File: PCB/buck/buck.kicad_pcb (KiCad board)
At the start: 2 copper layers, 30 x 27 mm, 7 parts, among them J1 UBat 38V, J2 Uout 5V, U1 LM2575-5.0BT

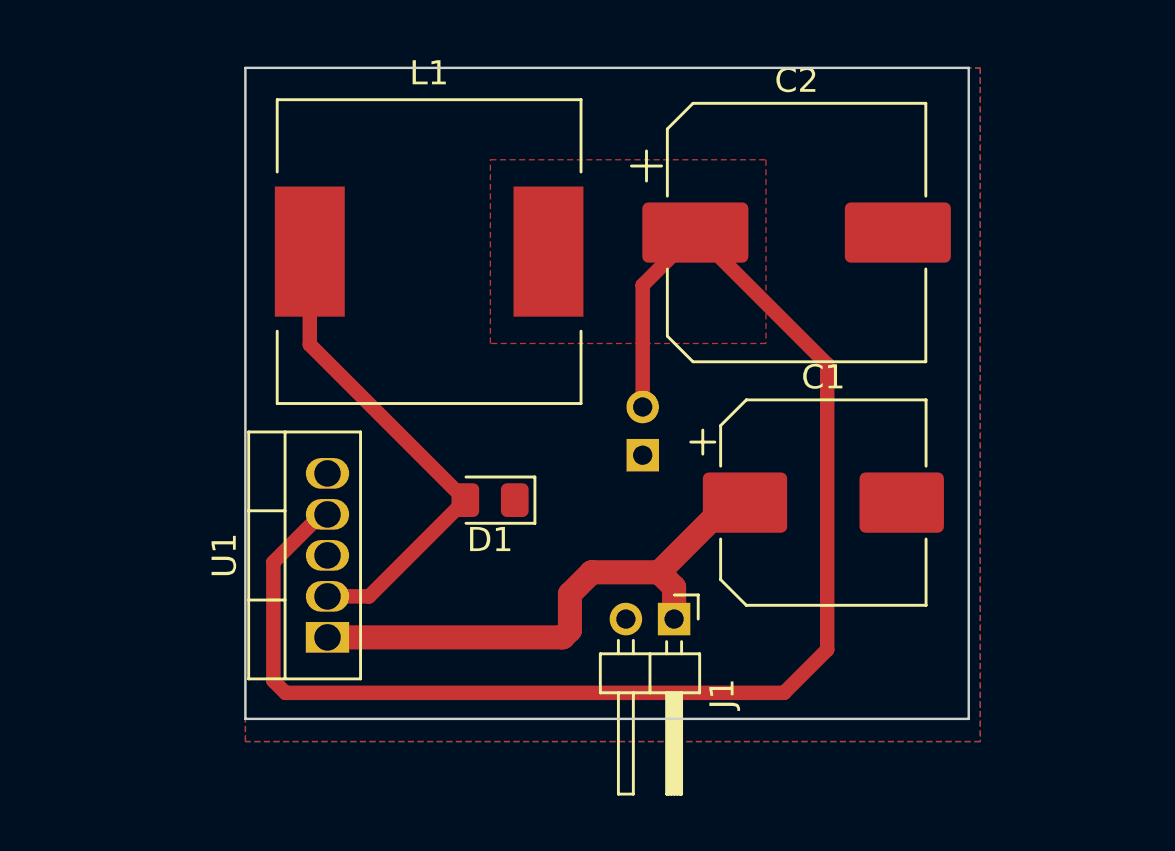
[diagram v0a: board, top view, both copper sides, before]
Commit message: Add files via upload
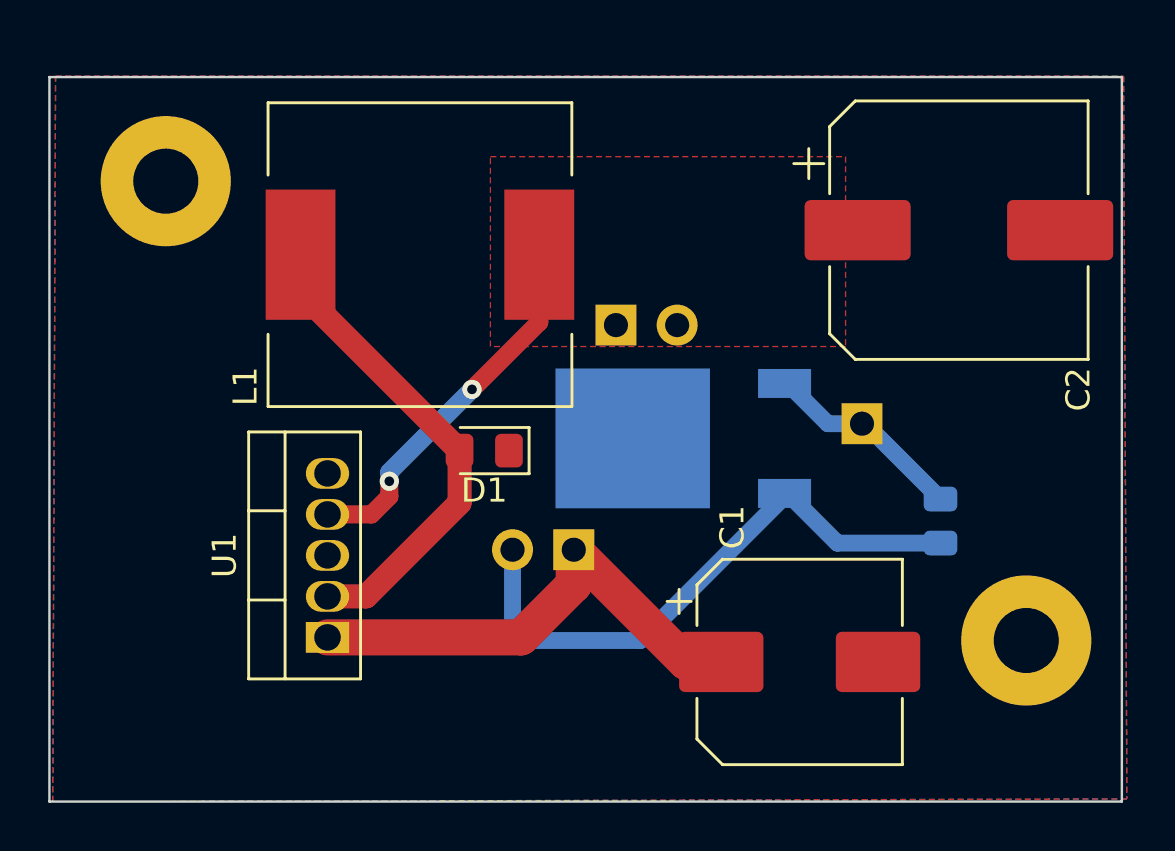
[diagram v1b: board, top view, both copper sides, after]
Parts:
- added H1: MountingHole_Pad, MountingHole:MountingHole_2.7mm_M2.5_Pad, F.Cu at (149.2, 105.0)
- added H2: MountingHole_Pad, MountingHole:MountingHole_2.7mm_M2.5_Pad, F.Cu at (113.5, 86.0)
- added J3: Zündung, Connector_PinSocket_2.54mm:PinSocket_1x01_P2.54mm_Horizontal, B.Cu at (142.4, 96.0)
- added Q1: QM6006D, Package_TO_SOT_SMD:TO-252-2, B.Cu at (135.0, 96.6)
- added R1: 100k, Resistor_SMD:R_0805_2012Metric, B.Cu at (145.7, 100.1)
- D1: value DIODE -> 1N4148
- J1: footprint Connector_PinHeader_2.00mm:PinHeader_1x02_P2.00mm_Horizontal -> Connector_PinSocket_2.54mm:PinSocket_1x02_P2.54mm_Horizontal; moved to B.Cu
- J2: footprint Connector_PinHeader_2.00mm:PinHeader_1x02_P2.00mm_Vertical -> Connector_PinSocket_2.54mm:PinSocket_1x02_P2.54mm_Horizontal
- moved C2 6.73 mm to (146.4, 88.0)
- moved C1 6.68 mm to (139.8, 105.9)
- moved J2 5.51 mm to (132.2, 91.9), turned to -90 degrees
- moved J1 5.06 mm to (130.5, 101.3), turned to 90 degrees
- moved D1 2.07 mm to (126.7, 97.2)
- moved L1 0.40 mm to (124.1, 89.0)
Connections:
- J1 pad 2: GND -> Net-(J1-Pad2)
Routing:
- net +5V: track 60.7 -> 15.5 mm, vias 0 -> 2
- net Net-(J1-Pad2): track 0.00 -> 24.6 mm
- net Net-(J3-Pad1): track 0.00 -> 8.33 mm
- net Net-(C1-Pad1): track 22.7 -> 20.6 mm
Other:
- board size 30 x 27 mm -> 44.5 x 30 mm
